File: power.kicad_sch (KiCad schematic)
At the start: 33 parts, among them J1 DC_Jack, Q1 FDD4243, U1 MAX17634BATP+, U2 TLV1117LV33DCYR

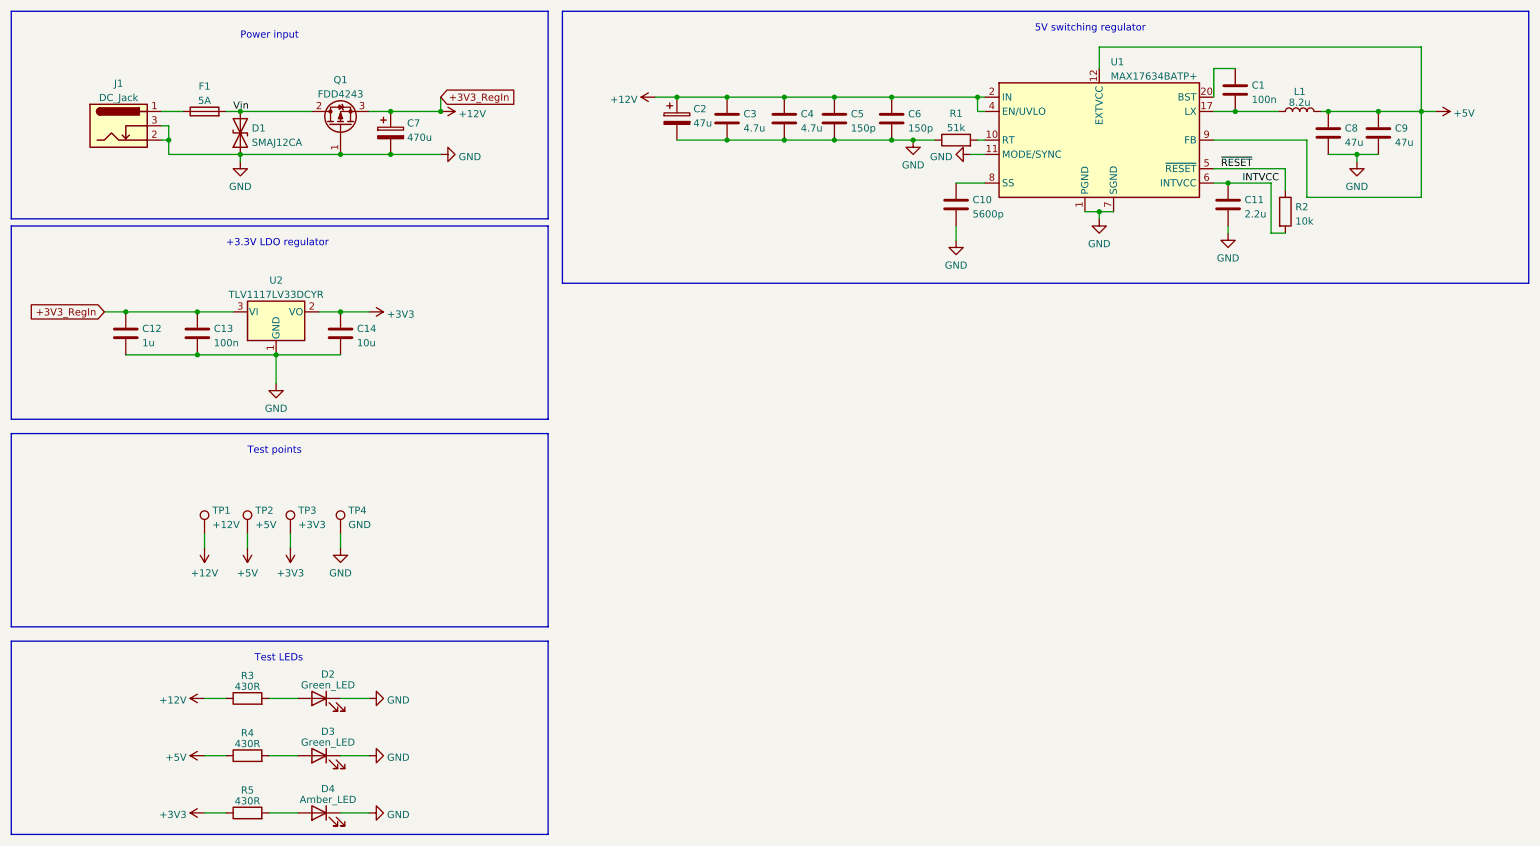
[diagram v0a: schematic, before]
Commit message: Fix third revision
Signed-off-by: Roman Ondráček <ondracek.roman@centrum.cz>
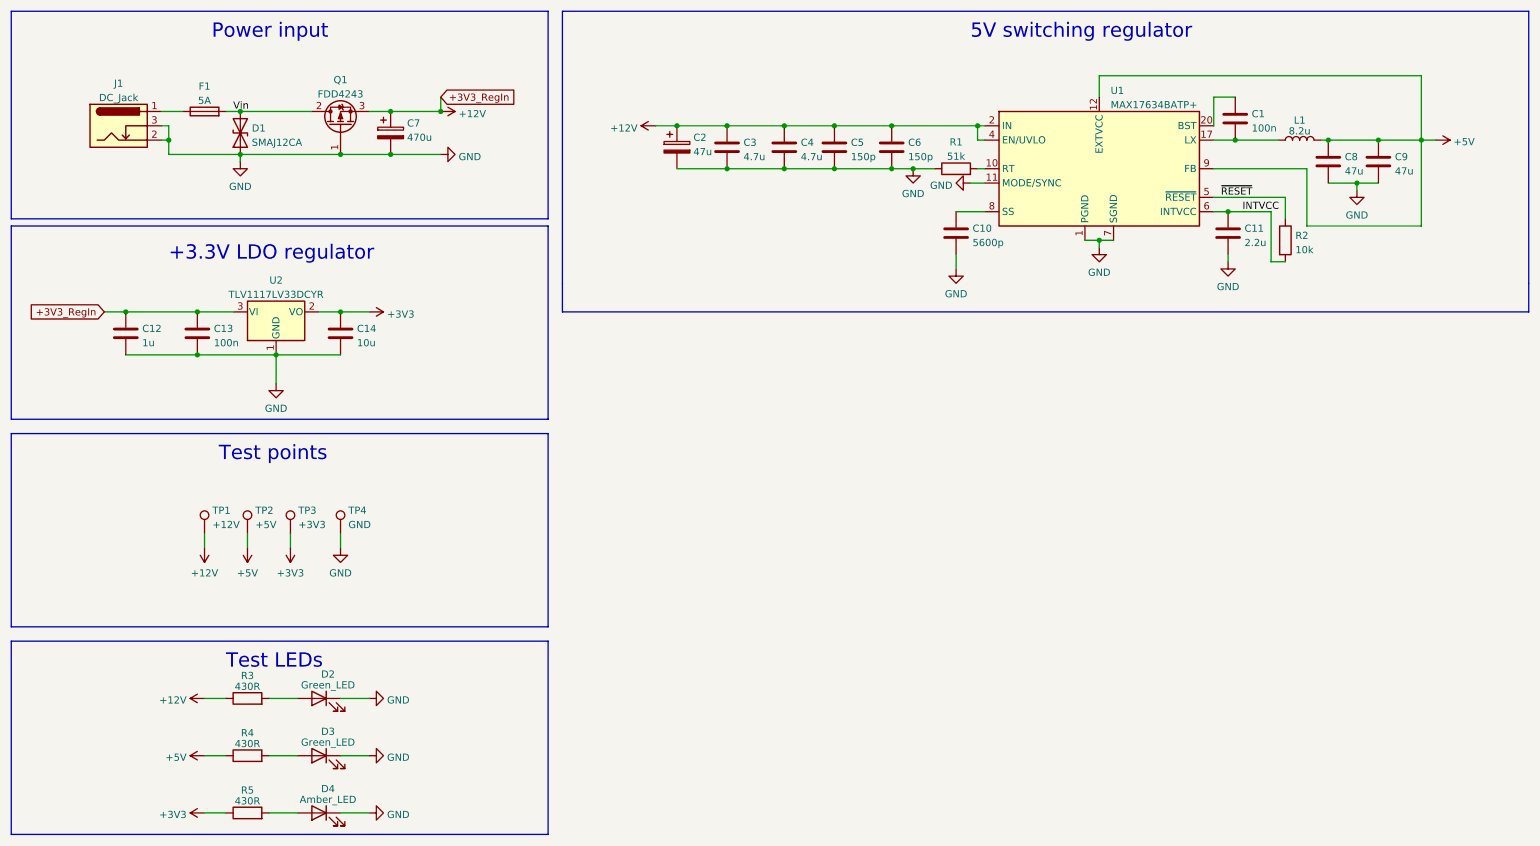
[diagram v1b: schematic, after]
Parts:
- C1, C13: Mouser https://cz.mouser.com/ProductDetail/187-CL21B104KCFSFNE -> https://cz.mouser.com/ProductDetail/81-GRM155R62A104KE4J
- C7: Mouser (none) -> https://cz.mouser.com/ProductDetail/647-UVR1C471MPD
- J1: Mouser https://cz.mouser.com/ProductDetail/161-0725-E -> (none); TME (none) -> https://www.tme.eu/cz/details/fc68148/konektory-dc/cliff/dc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
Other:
- moved on the sheet: C1, C10, C11, C2, C3, C4, C5, C6, C8, C9, L1, R1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
